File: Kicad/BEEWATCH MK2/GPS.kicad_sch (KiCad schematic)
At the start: 12 parts, among them U3 MPU-6050

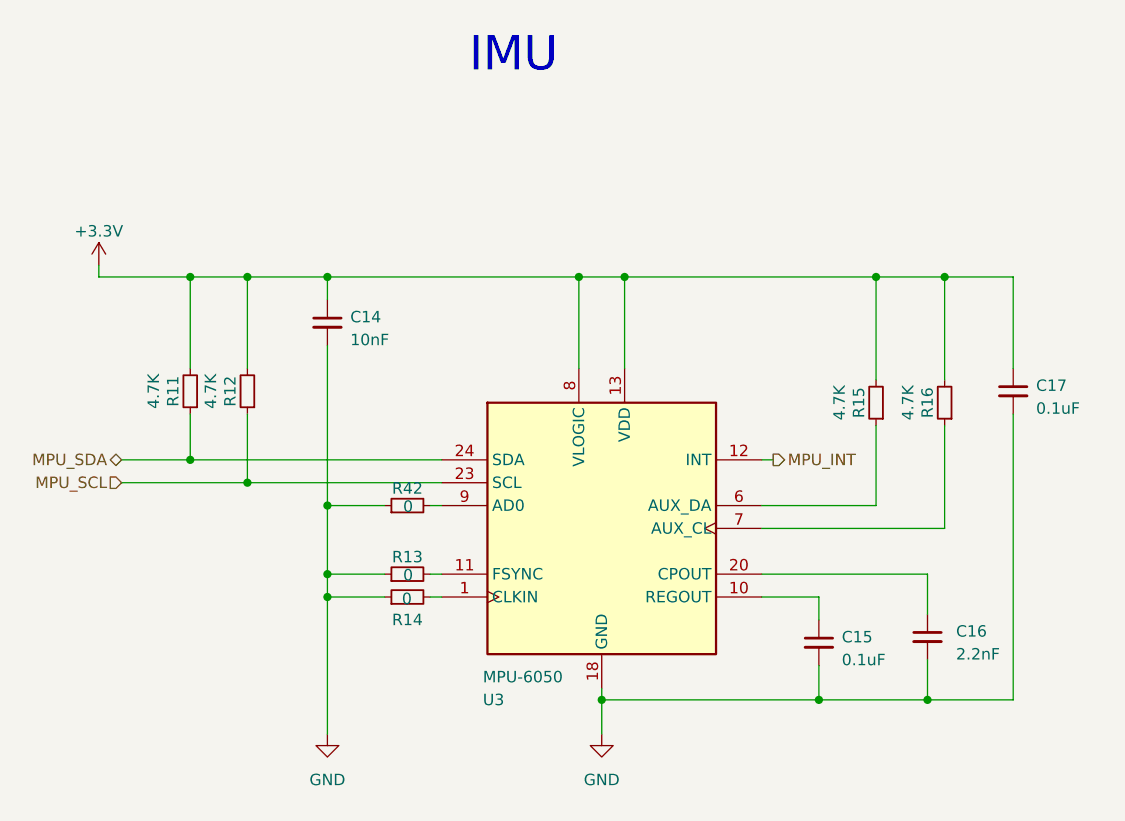
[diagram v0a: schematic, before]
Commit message: ERC Checking
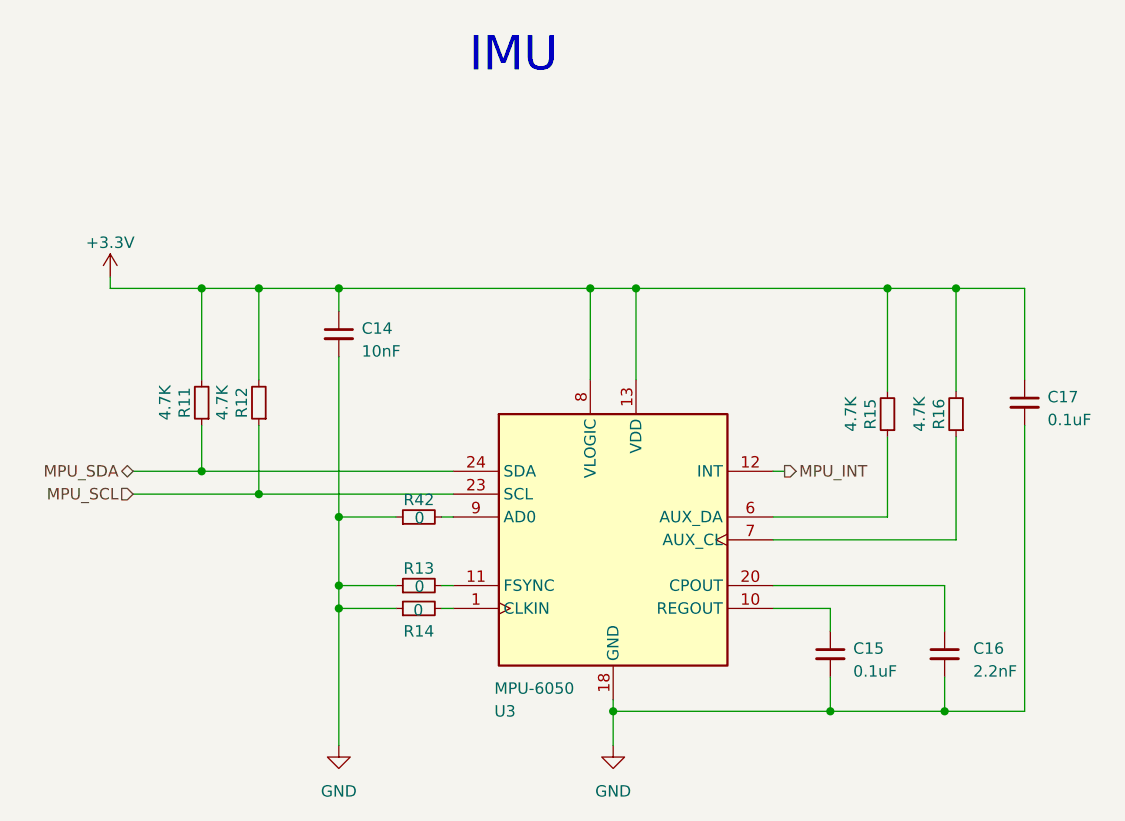
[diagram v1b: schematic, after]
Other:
- moved on the sheet: C14, C15, C16, C17, R11, R12, R13, R14, R15, R16, R42, U3
